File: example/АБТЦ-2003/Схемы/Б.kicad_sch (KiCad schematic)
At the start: 30 parts

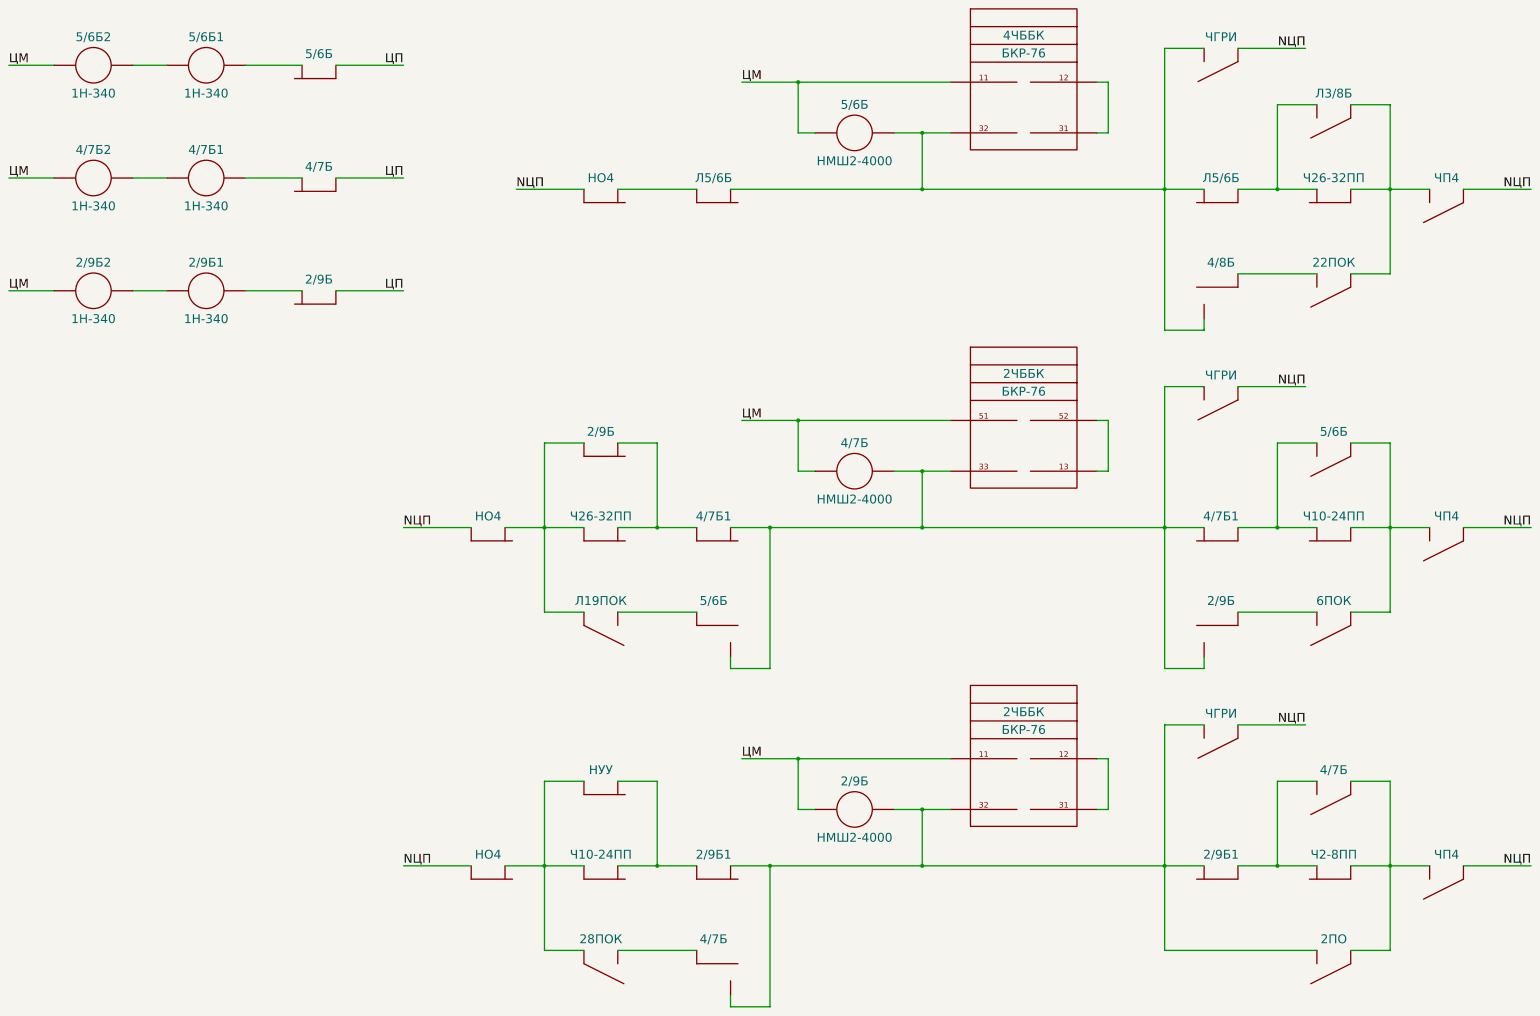
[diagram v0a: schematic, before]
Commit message: Шаблон АБТЦ обновлен
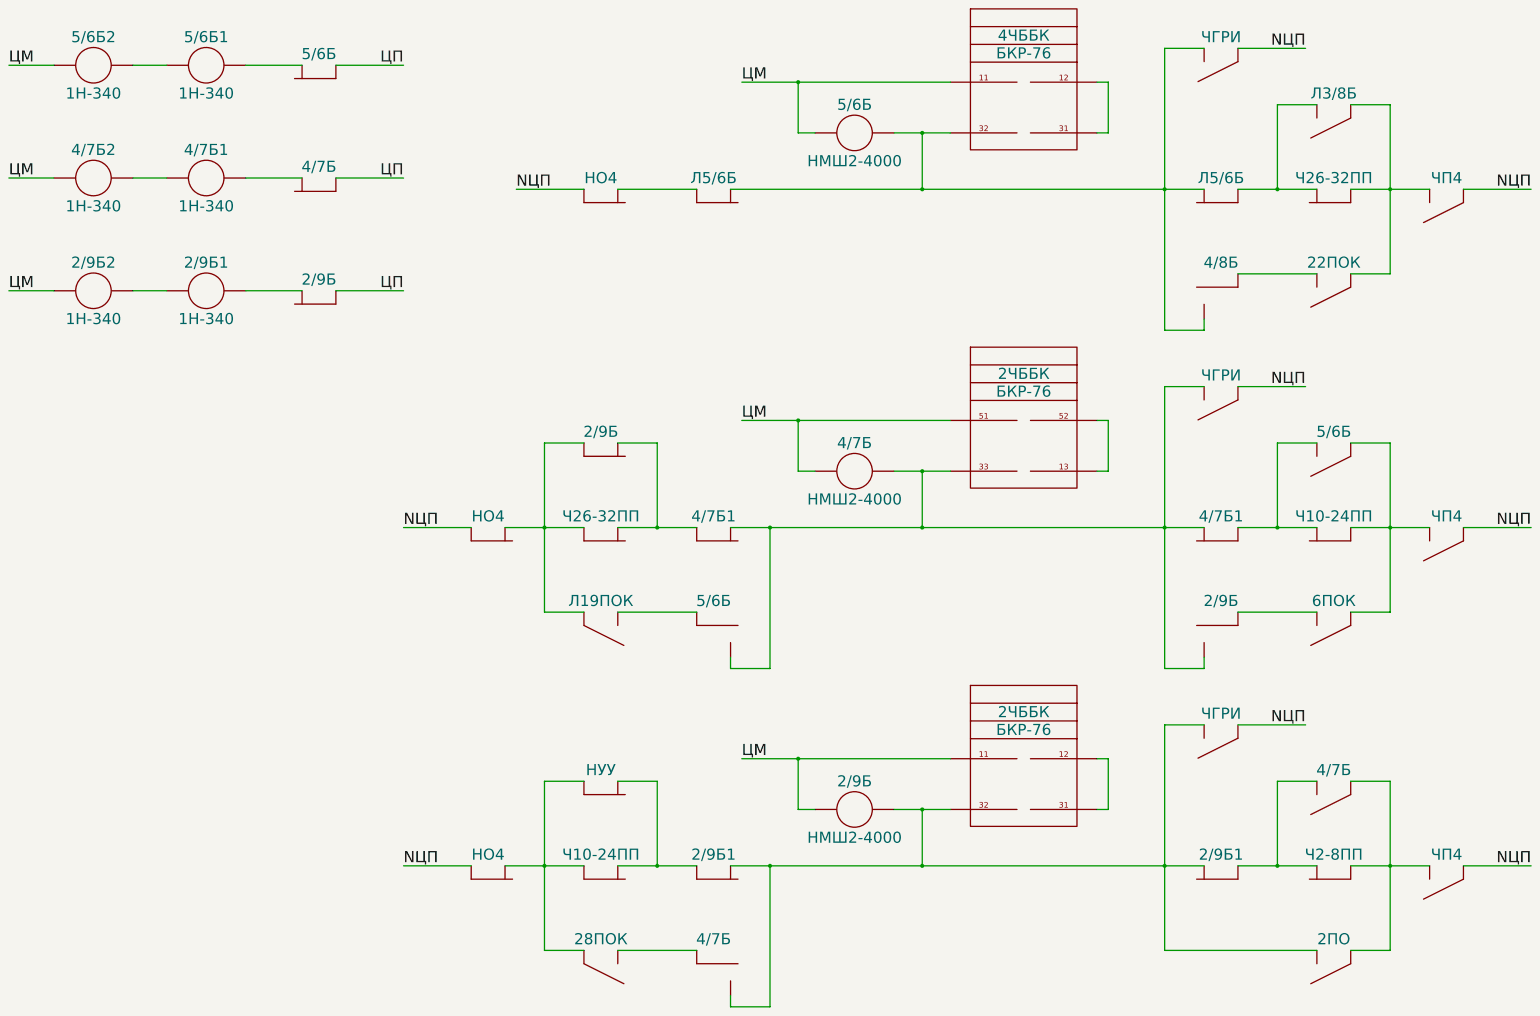
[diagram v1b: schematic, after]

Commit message: Обновление примера
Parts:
- Н1, Н11, Н111, Н1111, Н11111, Н1112, Н11121: symbol SCB_Relay:Контакт_нейтрального_якоря -> SCB_Legacy:Контакт_нейтрального_якоря_бн
- Н1, Н12, Н121, Н1211, Н12111, Н121111, Н1211111, Н12111111, Н121112, Н121113, Н12112, Н13: symbol SCB_Relay:Контакт_нейтрального_якоря_НЗ -> SCB_Legacy:Контакт_нейтрального_якоря_НЗ_бн
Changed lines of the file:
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@@
 (kicad_sch
-	(version 20231120)
+	(version 20250114)
 	(generator "eeschema")
-	(generator_version "8.0")
+	(generator_version "9.0")
 	(paper "A3")
 	(title_block
@@
 	)
 	(symbol
-		(lib_id "SCB_Relay:Контакт_нейтрального_якоря")
+		(lib_name "Контакт_нейтрального_якоря_бн_10")
+		(lib_id "SCB_Legacy:Контакт_нейтрального_якоря_бн")
 		(at 361.95 218.44 0)
 		(mirror y)
@@
 	)
 	(symbol
-		(lib_name "SCB_Relay:Контакт_нейтрального_якоря")
-		(lib_id "SCB_Relay:Контакт_нейтрального_якоря")
+		(lib_name "Контакт_нейтрального_якоря_бн_11")
+		(lib_id "SCB_Legacy:Контакт_нейтрального_якоря_бн")
 		(at 336.55 199.39 0)
 		(mirror y)
@@
 	)
 	(symbol
-		(lib_name "SCB_Relay:Контакт_нейтрального_якоря")
-		(lib_id "SCB_Relay:Контакт_нейтрального_якоря")
+		(lib_name "Контакт_нейтрального_якоря_бн_12")
+		(lib_id "SCB_Legacy:Контакт_нейтрального_якоря_бн")
 		(at 171.45 161.29 0)
 		(unit 3)
@@
 	)
 	(symbol
-		(lib_id "SCB_Relay:Контакт_нейтрального_якоря_НЗ")
+		(lib_name "Контакт_нейтрального_якоря_НЗ_бн_4")
+		(lib_id "SCB_Legacy:Контакт_нейтрального_якоря_НЗ_бн")
 		(at 336.55 142.24 0)
 		(mirror y)
@@
 	)
 	(symbol
-		(lib_name "SCB_Relay:Контакт_нейтрального_якоря")
-		(lib_id "SCB_Relay:Контакт_нейтрального_якоря")
+		(lib_name "Контакт_нейтрального_якоря_бн_8")
+		(lib_id "SCB_Legacy:Контакт_нейтрального_якоря_бн")
 		(at 311.15 34.29 0)
 		(mirror y)
@@
 	)
 	(symbol
-		(lib_name "SCB_Relay:Контакт_нейтрального_якоря")
-		(lib_id "SCB_Relay:Контакт_нейтрального_якоря")
+		(lib_name "Контакт_нейтрального_якоря_бн_6")
+		(lib_id "SCB_Legacy:Контакт_нейтрального_якоря_бн")
 		(at 361.95 142.24 0)
 		(mirror y)
@@
 	)
 	(symbol
-		(lib_name "SCB_Relay:Контакт_нейтрального_якоря_НЗ")
-		(lib_id "SCB_Relay:Контакт_нейтрального_якоря_НЗ")
+		(lib_name "Контакт_нейтрального_якоря_НЗ_бн_11")
+		(lib_id "SCB_Legacy:Контакт_нейтрального_якоря_НЗ_бн")
 		(at 311.15 142.24 0)
 		(mirror y)
@@
 	)
 	(symbol
-		(lib_name "SCB_Relay:Контакт_нейтрального_якоря_НЗ")
-		(lib_id "SCB_Relay:Контакт_нейтрального_якоря_НЗ")
+		(lib_name "Контакт_нейтрального_якоря_НЗ_бн_9")
+		(lib_id "SCB_Legacy:Контакт_нейтрального_якоря_НЗ_бн")
 		(at 196.85 66.04 0)
 		(unit 3)
@@
 	)
 	(symbol
-		(lib_name "SCB_Relay:Контакт_нейтрального_якоря_НЗ")
-		(lib_id "SCB_Relay:Контакт_нейтрального_якоря_НЗ")
+		(lib_name "Контакт_нейтрального_якоря_НЗ_бн_20")
+		(lib_id "SCB_Legacy:Контакт_нейтрального_якоря_НЗ_бн")
 		(at 171.45 199.39 0)
 		(unit 3)
@@
 	)
 	(symbol
-		(lib_name "SCB_Relay:Контакт_нейтрального_якоря_НЗ")
-		(lib_id "SCB_Relay:Контакт_нейтрального_якоря_НЗ")
+		(lib_name "Контакт_нейтрального_якоря_НЗ_бн_7")
+		(lib_id "SCB_Legacy:Контакт_нейтрального_якоря_НЗ_бн")
 		(at 196.85 142.24 0)
 		(unit 3)
@@
 	)
 	(symbol
-		(lib_name "SCB_Relay:Контакт_нейтрального_якоря_НЗ")
-		(lib_id "SCB_Relay:Контакт_нейтрального_якоря_НЗ")
+		(lib_name "Контакт_нейтрального_якоря_НЗ_бн_19")
+		(lib_id "SCB_Legacy:Контакт_нейтрального_якоря_НЗ_бн")
 		(at 171.45 123.19 0)
 		(unit 3)
@@
 	)
 	(symbol
-		(lib_name "SCB_Relay:Контакт_нейтрального_якоря_НЗ")
-		(lib_id "SCB_Relay:Контакт_нейтрального_якоря_НЗ")
+		(lib_name "Контакт_нейтрального_якоря_НЗ_бн_22")
+		(lib_id "SCB_Legacy:Контакт_нейтрального_якоря_НЗ_бн")
 		(at 146.05 218.44 0)
 		(unit 3)
@@
 	)
 	(symbol
-		(lib_name "SCB_Relay:Контакт_нейтрального_якоря")
-		(lib_id "SCB_Relay:Контакт_нейтрального_якоря")
+		(lib_id "SCB_Legacy:Контакт_нейтрального_якоря_бн")
 		(at 336.55 237.49 0)
 		(mirror y)
@@
 	)
 	(symbol
-		(lib_name "SCB_Relay:Контакт_нейтрального_якоря_НЗ")
-		(lib_id "SCB_Relay:Контакт_нейтрального_якоря_НЗ")
+		(lib_name "Контакт_нейтрального_якоря_НЗ_бн_12")
+		(lib_id "SCB_Legacy:Контакт_нейтрального_якоря_НЗ_бн")
 		(at 336.55 218.44 0)
 		(mirror y)
@@
 	)
 	(symbol
-		(lib_name "SCB_Relay:Контакт_нейтрального_якоря")
-		(lib_id "SCB_Relay:Контакт_нейтрального_якоря")
+		(lib_name "Контакт_нейтрального_якоря_бн_9")
+		(lib_id "SCB_Legacy:Контакт_нейтрального_якоря_бн")
 		(at 336.55 85.09 0)
 		(mirror y)
@@
 	)
 	(symbol
-		(lib_name "SCB_Relay:Контакт_нейтрального_якоря_НЗ")
-		(lib_id "SCB_Relay:Контакт_нейтрального_якоря_НЗ")
+		(lib_name "Контакт_нейтрального_якоря_НЗ_бн_17")
+		(lib_id "SCB_Legacy:Контакт_нейтрального_якоря_НЗ_бн")
 		(at 311.15 85.09 0)
 		(mirror y)
@@
 	)
 	(symbol
-		(lib_name "SCB_Relay:Контакт_нейтрального_якоря_НЗ")
-		(lib_id "SCB_Relay:Контакт_нейтрального_якоря_НЗ")
+		(lib_name "Контакт_нейтрального_якоря_НЗ_бн_1")
+		(lib_id "SCB_Legacy:Контакт_нейтрального_якоря_НЗ_бн")
 		(at 107.95 63.5 0)
 		(mirror y)
@@
 	)
 	(symbol
-		(lib_name "SCB_Relay:Контакт_нейтрального_якоря_НЗ")
-		(lib_id "SCB_Relay:Контакт_нейтрального_якоря_НЗ")
+		(lib_name "Контакт_нейтрального_якоря_НЗ_бн_8")
+		(lib_id "SCB_Legacy:Контакт_нейтрального_якоря_НЗ_бн")
 		(at 311.15 66.04 0)
 		(mirror y)
@@
 	)
 	(symbol
-		(lib_name "SCB_Relay:Контакт_нейтрального_якоря_НЗ")
-		(lib_id "SCB_Relay:Контакт_нейтрального_якоря_НЗ")
+		(lib_name "Контакт_нейтрального_якоря_НЗ_бн_18")
+		(lib_id "SCB_Legacy:Контакт_нейтрального_якоря_НЗ_бн")
 		(at 311.15 161.29 0)
 		(mirror y)
@@
 	)
 	(symbol
-		(lib_name "SCB_Relay:Контакт_нейтрального_якоря_НЗ")
-		(lib_id "SCB_Relay:Контакт_нейтрального_якоря_НЗ")
+		(lib_name "Контакт_нейтрального_якоря_НЗ_бн_14")
+		(lib_id "SCB_Legacy:Контакт_нейтрального_якоря_НЗ_бн")
 		(at 336.55 66.04 0)
 		(mirror y)
@@
 	)
 	(symbol
-		(lib_name "SCB_Relay:Контакт_нейтрального_якоря_НЗ")
-		(lib_id "SCB_Relay:Контакт_нейтрального_якоря_НЗ")
+		(lib_name "Контакт_нейтрального_якоря_НЗ_бн_10")
+		(lib_id "SCB_Legacy:Контакт_нейтрального_якоря_НЗ_бн")
 		(at 171.45 142.24 0)
 		(unit 3)
@@
 	)
 	(symbol
-		(lib_name "SCB_Relay:Контакт_нейтрального_якоря")
-		(lib_id "SCB_Relay:Контакт_нейтрального_якоря")
+		(lib_name "Контакт_нейтрального_якоря_бн_1")
+		(lib_id "SCB_Legacy:Контакт_нейтрального_якоря_бн")
 		(at 171.45 237.49 0)
 		(unit 3)
@@
 	)
 	(symbol
-		(lib_name "SCB_Relay:Контакт_нейтрального_якоря_НЗ")
-		(lib_id "SCB_Relay:Контакт_нейтрального_якоря_НЗ")
+		(lib_id "SCB_Legacy:Контакт_нейтрального_якоря_НЗ_бн")
 		(at 196.85 161.29 0)
 		(unit 2)
@@
 	)
 	(symbol
-		(lib_name "SCB_Relay:Контакт_нейтрального_якоря_НЗ")
-		(lib_id "SCB_Relay:Контакт_нейтрального_якоря_НЗ")
+		(lib_name "Контакт_нейтрального_якоря_НЗ_бн_3")
+		(lib_id "SCB_Legacy:Контакт_нейтрального_якоря_НЗ_бн")
 		(at 196.85 237.49 0)
 		(unit 2)
@@
 	)
 	(symbol
-		(lib_name "SCB_Relay:Контакт_нейтрального_якоря_НЗ")
-		(lib_id "SCB_Relay:Контакт_нейтрального_якоря_НЗ")
+		(lib_name "Контакт_нейтрального_якоря_НЗ_бн_5")
+		(lib_id "SCB_Legacy:Контакт_нейтрального_якоря_НЗ_бн")
 		(at 171.45 66.04 0)
 		(unit 3)
@@
 	)
 	(symbol
-		(lib_name "SCB_Relay:Контакт_нейтрального_якоря_НЗ")
-		(lib_id "SCB_Relay:Контакт_нейтрального_якоря_НЗ")
+		(lib_name "Контакт_нейтрального_якоря_НЗ_бн_15")
+		(lib_id "SCB_Legacy:Контакт_нейтрального_якоря_НЗ_бн")
 		(at 171.45 218.44 0)
 		(unit 3)
@@
 	)
 	(symbol
-		(lib_name "SCB_Relay:Контакт_нейтрального_якоря")
-		(lib_id "SCB_Relay:Контакт_нейтрального_якоря")
+		(lib_name "Контакт_нейтрального_якоря_бн_13")
+		(lib_id "SCB_Legacy:Контакт_нейтрального_якоря_бн")
 		(at 311.15 186.69 0)
 		(mirror y)
@@
 	)
 	(symbol
-		(lib_name "SCB_Relay:Контакт_нейтрального_якоря")
-		(lib_id "SCB_Relay:Контакт_нейтрального_якоря")
+		(lib_name "Контакт_нейтрального_якоря_бн_5")
+		(lib_id "SCB_Legacy:Контакт_нейтрального_якоря_бн")
 		(at 336.55 161.29 0)
 		(mirror y)
@@
 	)
 	(symbol
-		(lib_name "SCB_Relay:Контакт_нейтрального_якоря_НЗ")
-		(lib_id "SCB_Relay:Контакт_нейтрального_якоря_НЗ")
+		(lib_name "Контакт_нейтрального_якоря_НЗ_бн_13")
+		(lib_id "SCB_Legacy:Контакт_нейтрального_якоря_НЗ_бн")
 		(at 196.85 218.44 0)
 		(unit 3)
@@
 	)
 	(symbol
-		(lib_name "SCB_Relay:Контакт_нейтрального_якоря")
-		(lib_id "SCB_Relay:Контакт_нейтрального_якоря")
+		(lib_name "Контакт_нейтрального_якоря_бн_7")
+		(lib_id "SCB_Legacy:Контакт_нейтрального_якоря_бн")
 		(at 311.15 110.49 0)
 		(mirror y)
@@
 	)
 	(symbol
-		(lib_name "SCB_Relay:Контакт_нейтрального_якоря")
-		(lib_id "SCB_Relay:Контакт_нейтрального_якоря")
+		(lib_name "Контакт_нейтрального_якоря_бн_3")
+		(lib_id "SCB_Legacy:Контакт_нейтрального_якоря_бн")
 		(at 336.55 46.99 0)
 		(mirror y)
@@
 	)
 	(symbol
-		(lib_name "SCB_Relay:Контакт_нейтрального_якоря_НЗ")
-		(lib_id "SCB_Relay:Контакт_нейтрального_якоря_НЗ")
+		(lib_name "Контакт_нейтрального_якоря_НЗ_бн_21")
+		(lib_id "SCB_Legacy:Контакт_нейтрального_якоря_НЗ_бн")
 		(at 107.95 38.1 0)
 		(mirror y)
@@
 	)
 	(symbol
-		(lib_name "SCB_Relay:Контакт_нейтрального_якоря_НЗ")
-		(lib_id "SCB_Relay:Контакт_нейтрального_якоря_НЗ")
+		(lib_name "Контакт_нейтрального_якоря_НЗ_бн_2")
+		(lib_id "SCB_Legacy:Контакт_нейтрального_якоря_НЗ_бн")
 		(at 107.95 88.9 0)
 		(mirror y)
@@
 	)
 	(symbol
-		(lib_name "SCB_Relay:Контакт_нейтрального_якоря")
-		(lib_id "SCB_Relay:Контакт_нейтрального_якоря")
+		(lib_name "Контакт_нейтрального_якоря_бн_4")
+		(lib_id "SCB_Legacy:Контакт_нейтрального_якоря_бн")
 		(at 361.95 66.04 0)
 		(mirror y)
@@
 	)
 	(symbol
-		(lib_name "SCB_Relay:Контакт_нейтрального_якоря")
-		(lib_id "SCB_Relay:Контакт_нейтрального_якоря")
+		(lib_name "Контакт_нейтрального_якоря_бн_2")
+		(lib_id "SCB_Legacy:Контакт_нейтрального_якоря_бн")
 		(at 336.55 123.19 0)
 		(mirror y)
@@
 	)
 	(symbol
-		(lib_name "SCB_Relay:Контакт_нейтрального_якоря_НЗ")
-		(lib_id "SCB_Relay:Контакт_нейтрального_якоря_НЗ")
+		(lib_name "Контакт_нейтрального_якоря_НЗ_бн_16")
+		(lib_id "SCB_Legacy:Контакт_нейтрального_якоря_НЗ_бн")
 		(at 146.05 142.24 0)
 		(unit 3)
@@
 	)
 	(symbol
-		(lib_name "SCB_Relay:Контакт_нейтрального_якоря_НЗ")
-		(lib_id "SCB_Relay:Контакт_нейтрального_якоря_НЗ")
+		(lib_name "Контакт_нейтрального_якоря_НЗ_бн_6")
+		(lib_id "SCB_Legacy:Контакт_нейтрального_якоря_НЗ_бн")
 		(at 311.15 218.44 0)
 		(mirror y)
